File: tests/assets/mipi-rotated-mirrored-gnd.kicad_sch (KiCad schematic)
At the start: 0 parts

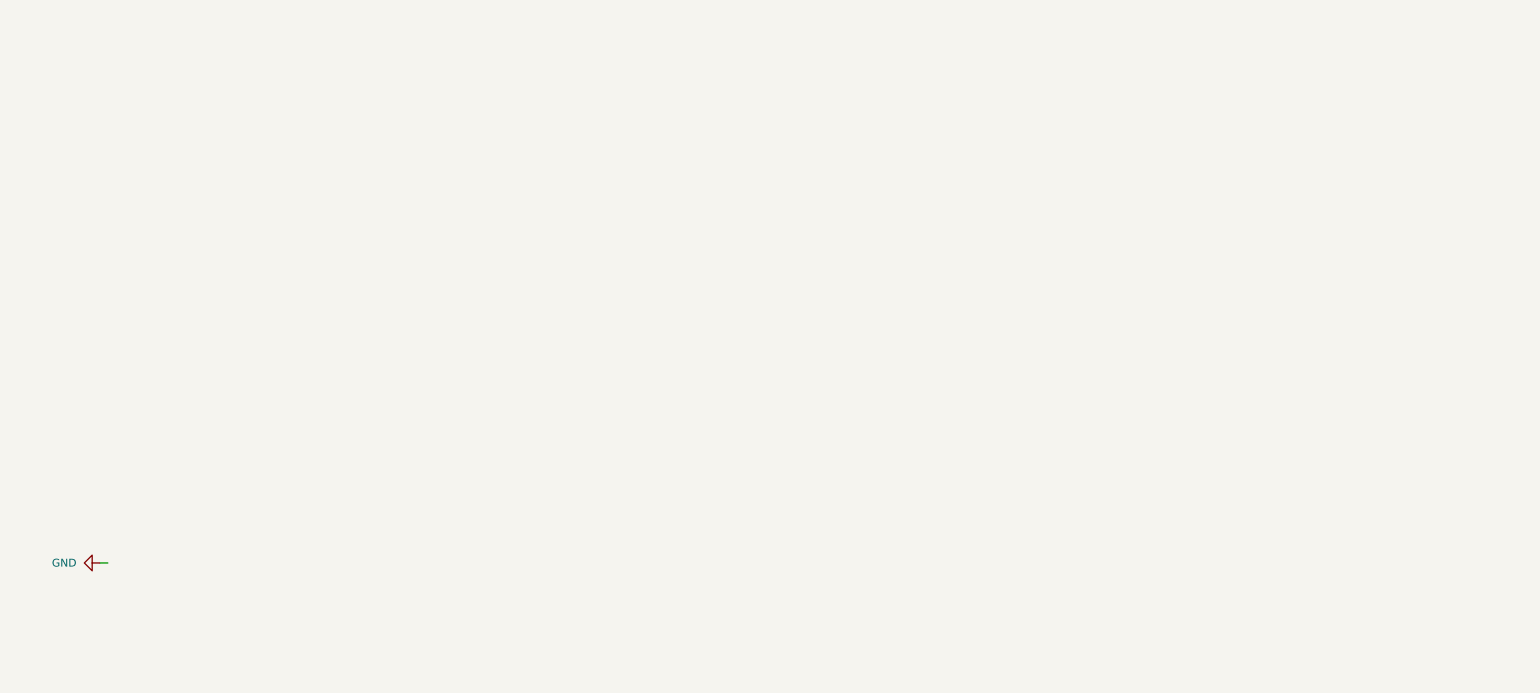
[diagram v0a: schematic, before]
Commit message: up
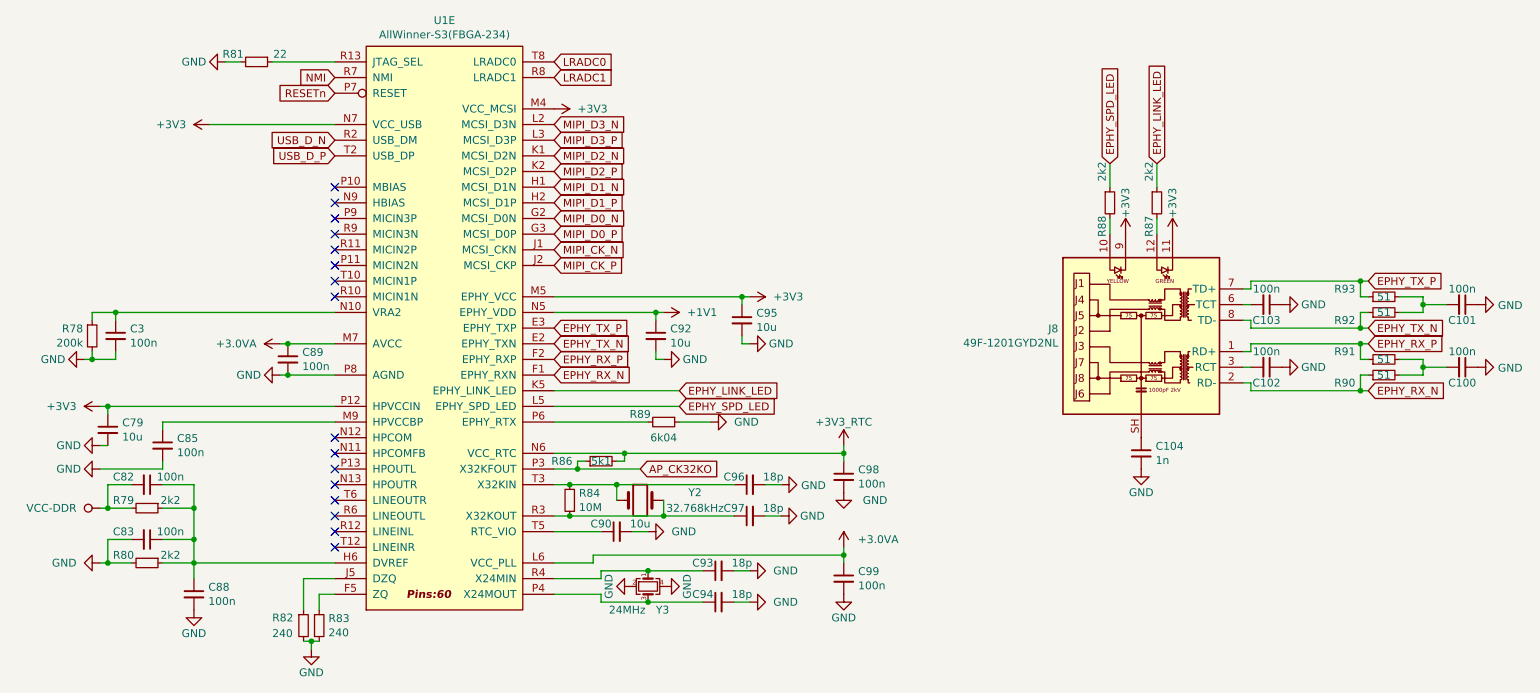
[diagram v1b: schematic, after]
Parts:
- added C100, C101, C102, C103, C3, C82, C83, C85, C88, C89, C98, C99: 100n, otter:C_0402, symbol Device:C_Small
- added C104: 1n, otter:C_0805, symbol Device:C_Small
- added C79, C90, C92, C95: 10u, otter:C_0603, symbol Device:C_Small
- added C93, C94, C96, C97: 18p, otter:C_0402, symbol Device:C_Small
- added J8: 49F-1201GYD2NL, otter:49F-1201GYDXNL, symbol otter:49F-1201GYD2NL
- added R78: 200k, otter:R_0402, symbol Device:R_Small
- added R79, R80, R87, R88: 2k2, otter:R_0402, symbol Device:R_Small
- added R81: 22, otter:R_0402, symbol Device:R_Small
- added R82, R83: 240, otter:R_0402, symbol Device:R_Small
- added R84: 10M, otter:R_0402, symbol Device:R_Small
- added R86: 5k1, otter:R_0402, symbol Device:R_Small
- added R89: 6k04, otter:R_0402, symbol Device:R_Small
- added R90, R91, R92, R93: 51, otter:R_0402, symbol Device:R_Small
- added U1: AllWinner-S3(FBGA-234), otter:FBGA-234(Pitch-0.65mm_Pad-0.3mm_11x11x1.08mm), symbol otter:AllWinner-S3(FBGA-234)
- added Y2: 32.768kHz, otter:Crystal_SMD_3215-2Pin_3.2x1.5mm, symbol Device:Crystal
- added Y3: 24MHz, otter:Oscillator_3225, symbol Device:Crystal_GND24_Small
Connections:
- net GND: now also C100.1, C101.1, C102.1, C103.1, C104.2, C3.2, C79.2, C83.2, C85.2, C88.2, C89.2, C90.2, C92.2, C93.2, C94.2, C95.2, C96.2, C97.2, C98.2, C99.2, R78.2, R80.2, R81.2, R82.2, R83.2, R89.1, U1.P8 (AGND), Y3.2, Y3.4
- new net: C3.1, R78.1, U1.N10 (VRA2)
- new net: J8.10, R88.2
- new net: J8.12, R87.2
- new net: C102.2, J8.3 (RCT)
- new net: C103.2, J8.6 (TCT)
- new net: C104.1, J8.SH
- new net: R83.1, U1.F5 (ZQ)
- new net: C82.1, C83.1, C88.1, R79.1, R80.1, U1.H6 (DVREF)
- new net: R82.1, U1.J5 (DZQ)
- new net: C85.1, U1.M9 (HPVCCBP)
- new net: C94.1, U1.P4 (X24MOUT), Y3.3
- new net: R89.2, U1.P6 (EPHY_RTX)
- new net: R81.1, U1.R13 (JTAG_SEL)
- new net: C97.1, R84.1, U1.R3 (X32KOUT), Y2.2
- new net: C93.1, U1.R4 (X24MIN), Y3.1
- new net: C96.1, R84.2, U1.T3 (X32KIN), Y2.1
- new net: C90.1, U1.T5 (RTC_VIO)
- new net: C100.2, R90.2, R91.2
- new net: C101.2, R92.2, R93.2
- new net +1V1: C92.1, U1.N5 (EPHY_VDD)
- new net +3.0VA: C89.1, C99.1, U1.L6 (VCC_PLL), U1.M7 (AVCC)
- new net +3.3V_RTC: C98.1, R86.2, U1.N6 (VCC_RTC)
- new net +3V3: C79.1, C95.1, J8.11, J8.9, U1.M4 (VCC_MCSI), U1.M5 (EPHY_VCC), U1.N7 (VCC_USB), U1.P12 (HPVCCIN)
- new net AP_CK32KO: R86.1, U1.P3 (X32KFOUT)
- new net EPHY_LINK_LED: R87.1, U1.K5 (EPHY_LINK_LED)
- new net EPHY_RX_N: J8.2 (RD-), R90.1, U1.F1 (EPHY_RXN)
- new net EPHY_RX_P: J8.1 (RD+), R91.1, U1.F2 (EPHY_RXP)
- new net EPHY_SPD_LED: R88.1, U1.L5 (EPHY_SPD_LED)
- new net EPHY_TX_N: J8.8 (TD-), R92.1, U1.E2 (EPHY_TXN)
- new net EPHY_TX_P: J8.7 (TD+), R93.1, U1.E3 (EPHY_TXP)
- new net LRADC0: U1.T8 (LRADC0)
- new net LRADC1: U1.R8 (LRADC1)
- new net MIPI_CK_N: U1.J1 (MCSI_CKN)
- new net MIPI_CK_P: U1.J2 (MCSI_CKP)
- new net MIPI_D0_N: U1.G2 (MCSI_D0N)
- new net MIPI_D0_P: U1.G3 (MCSI_D0P)
- new net MIPI_D1_N: U1.H1 (MCSI_D1N)
- new net MIPI_D1_P: U1.H2 (MCSI_D1P)
- new net MIPI_D2_N: U1.K1 (MCSI_D2N)
- new net MIPI_D2_P: U1.K2 (MCSI_D2P)
- new net MIPI_D3_N: U1.L2 (MCSI_D3N)
- new net MIPI_D3_P: U1.L3 (MCSI_D3P)
- new net NMI: U1.R7 (NMI)
- new net RESETn: U1.P7 (RESET)
- new net USB_D_N: U1.R2 (USB_DM)
- new net USB_D_P: U1.T2 (USB_DP)
- new net VCC-DDR: C82.2, R79.2
- no-connect marks 0 -> 16
